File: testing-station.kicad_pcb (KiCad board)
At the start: 4 copper layers, 95 x 53.9 mm, 83 parts, among them IC1 BME680, IC2 DS3231, IC3 74HC4050D, J1 pyranometer, J10 Conn_01x06_Socket, J11 Conn_01x08_Socket, J13 microSD, J2 anemometer, J3 AM2315C, J4 FPC connector, J5 Pt100, J6 Conn_01x10_Socket, J7 Pt100, J8 Conn_01x08_Socket, J9 Pt100, Q1 BSS138, SW1 500SSP1S2M2QEA, U1 TBA_1-0519, U2 MAX31865, U4 MAX31865, U6 MAX31865

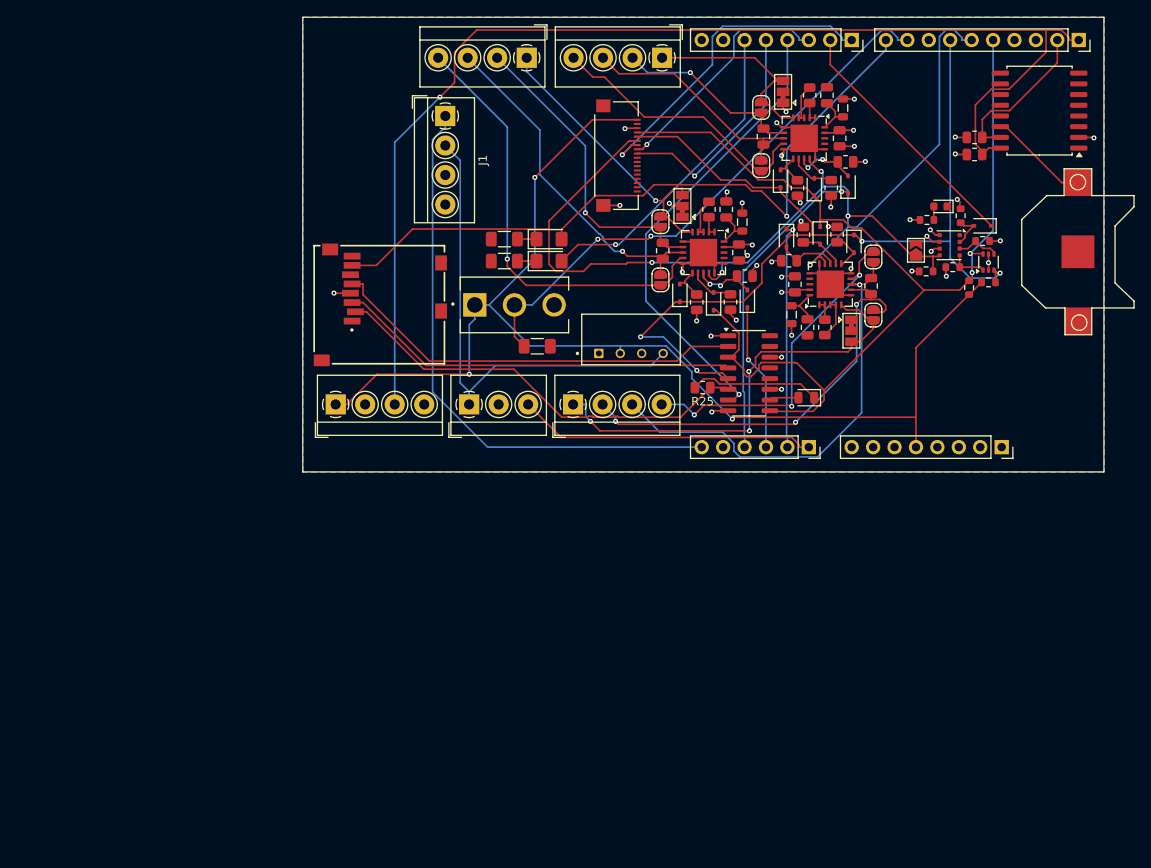
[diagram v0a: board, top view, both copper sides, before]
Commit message: more compact format
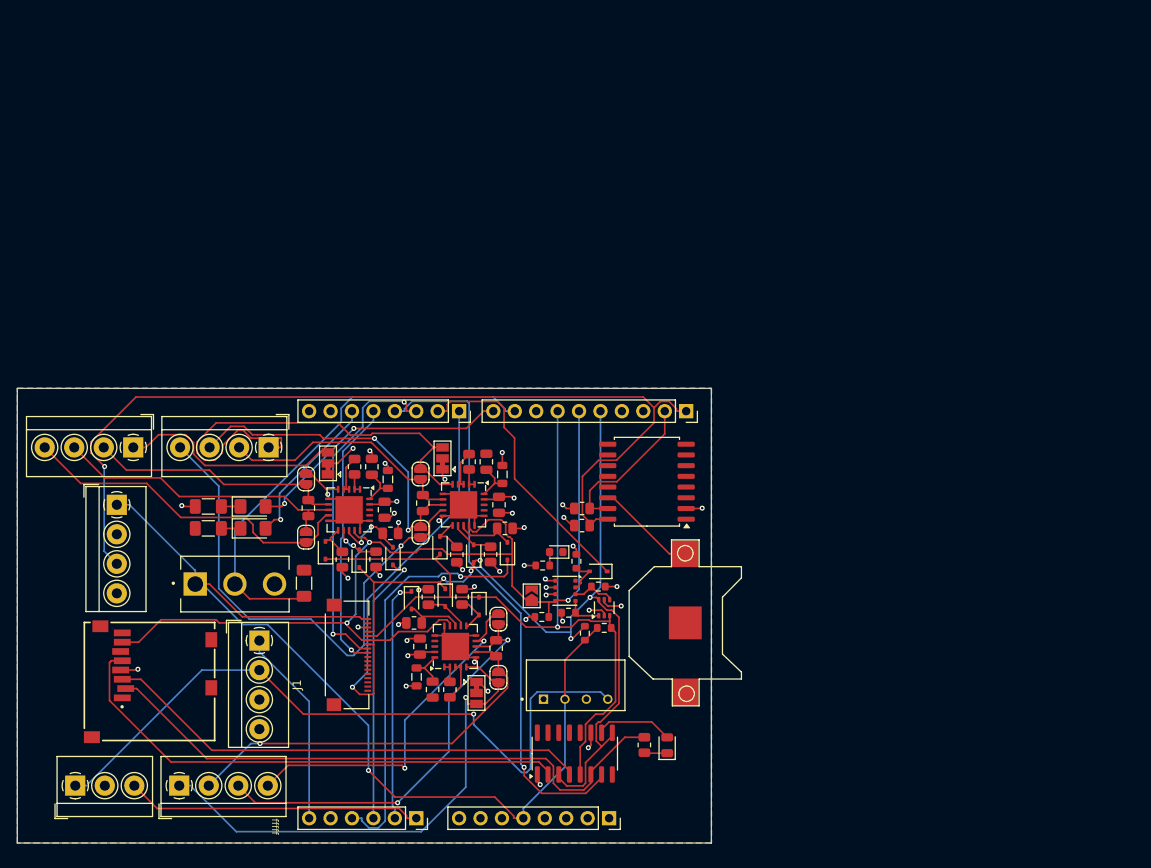
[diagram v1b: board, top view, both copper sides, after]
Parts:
- moved J4 67.3 mm to (155.1, 108.5)
- moved J1 66.0 mm to (144.7, 106.8)
- moved J9 65.6 mm to (145.8, 83.9)
- moved J7 65.6 mm to (129.7, 83.9)
- moved J2 65.0 mm to (122.8, 124.0)
- moved J5 65.0 mm to (135.2, 124.0)
- moved IC2 64.0 mm to (190.6, 88.0)
- moved J10 64.0 mm to (163.3, 127.9)
- moved J6 64.0 mm to (195.3, 79.6)
- moved B1 64.0 mm to (195.2, 104.7)
- moved J11 64.0 mm to (186.1, 127.9)
- moved J8 64.0 mm to (168.3, 79.6)
- moved R23 64.0 mm to (182.9, 93.2)
- moved R24 64.0 mm to (182.9, 91.1)
- moved C2 61.8 mm to (165.2, 112.6)
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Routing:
- net /A5: track 68.1 -> 23.6 mm
- net /MISO: track 153.1 -> 119.2 mm, vias 5 -> 3
- net Net-(J9-Pin_1): track 23.6 -> 55.7 mm
- net /SCL: track 142.6 -> 111.4 mm
- net Net-(J9-Pin_4): track 32.6 -> 60.7 mm, vias 0 -> 1
- net +9V: track 56.8 -> 83.8 mm, vias 0 -> 1
- net /SCK: track 128.5 -> 102.9 mm, vias 2 -> 5
- net /D8: track 57.3 -> 32.1 mm, vias 1 -> 2
- net +5V: track 140.4 -> 116.6 mm, vias 3 -> 1
- net /microSD/3Y: track 51.1 -> 71.1 mm
- net /MOSI: track 117.9 -> 98.5 mm, vias 4 -> 1
- net /D2: track 38.0 -> 18.7 mm
- net /A2: track 17.4 -> 32.6 mm
- net Net-(D14-K): track 15.5 -> 2.73 mm
- net /D4: track 55.1 -> 67.6 mm
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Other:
- board size 95 x 53.9 mm -> 82.3 x 53.9 mm
- board text added: "fffff"
